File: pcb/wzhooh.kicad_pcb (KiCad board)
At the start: 2 copper layers, 1 part, among them U1 Pico

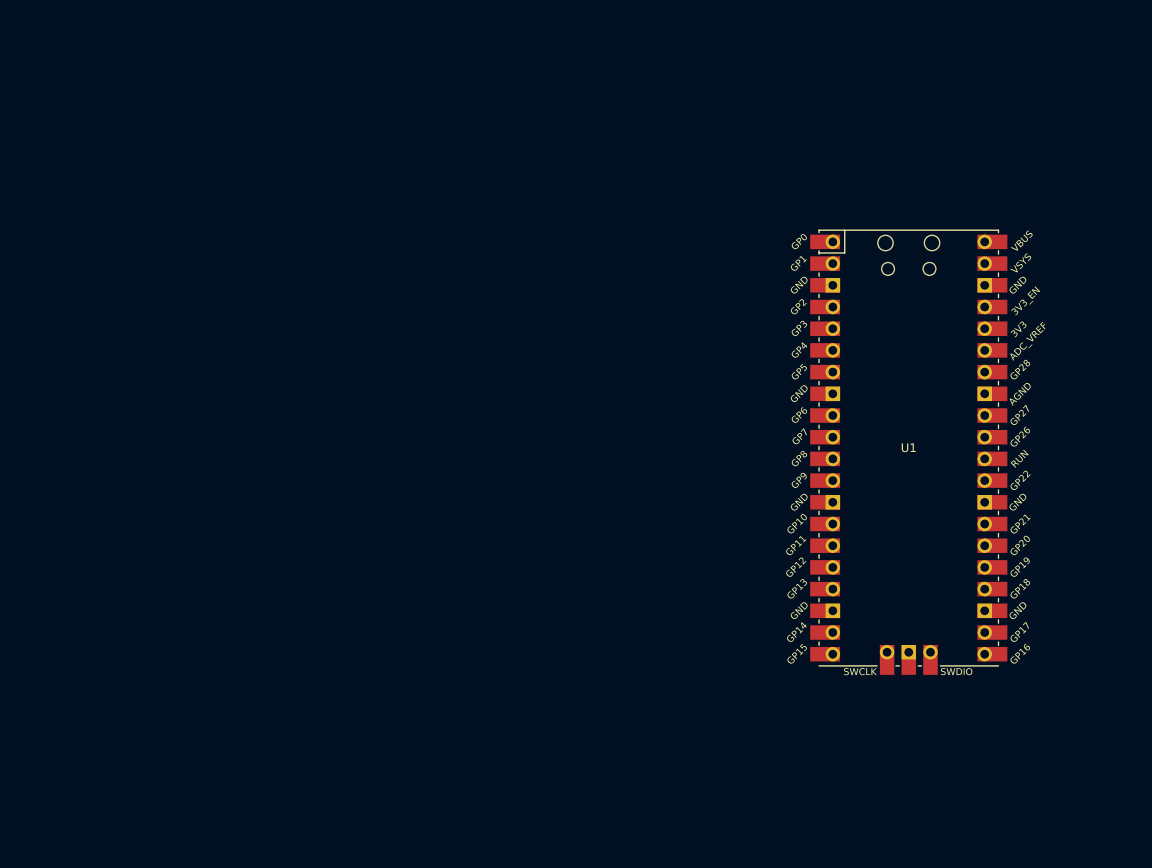
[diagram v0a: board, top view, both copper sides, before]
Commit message: rename project
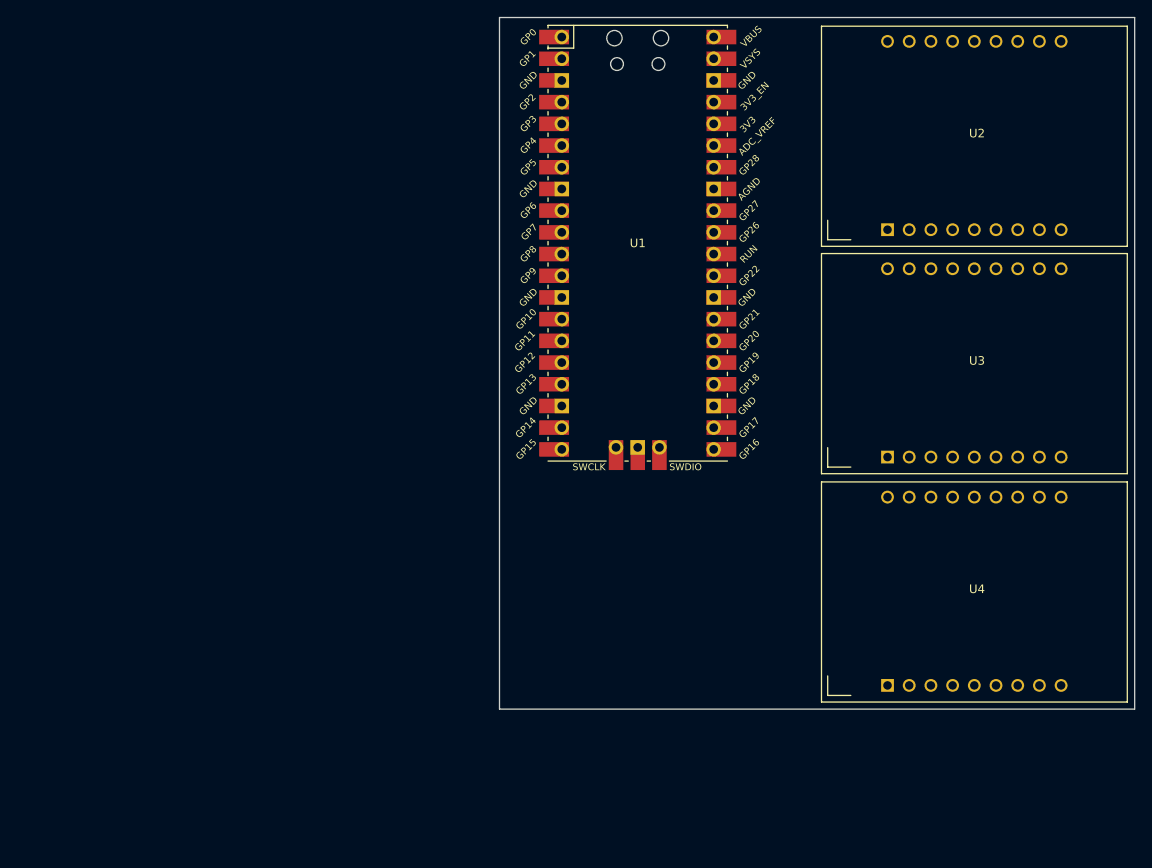
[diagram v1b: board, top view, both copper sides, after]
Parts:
- added U2: DA08-11SURKWA, Library:DA08-11, F.Cu at (150.1, 52.8)
- added U3: DA08-11SURKWA, Library:DA08-11, F.Cu at (150.1, 79.4)
- added U4: DA08-11SURKWA, Library:DA08-11, F.Cu at (150.1, 106.2)
- moved U1 39.8 mm to (110.7, 65.8)
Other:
- board outline added: 74.3 x 80.9 mm

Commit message: pcb rev:0x01
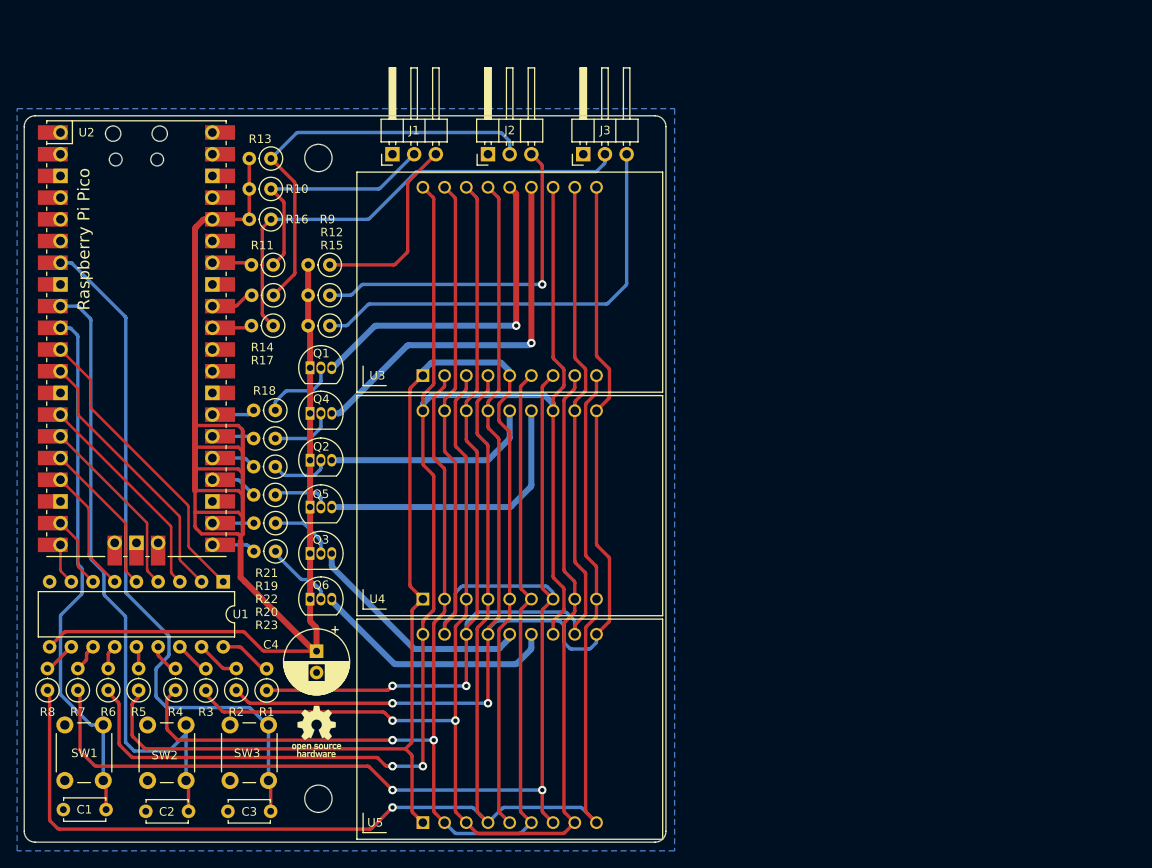
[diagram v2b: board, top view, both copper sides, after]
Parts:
- added C1: 1nF, Capacitor_THT:C_Disc_D4.7mm_W2.5mm_P5.00mm, F.Cu at (48.5, 132.1)
- added C2: 1nF, Capacitor_THT:C_Disc_D4.7mm_W2.5mm_P5.00mm, F.Cu at (58.2, 132.3)
- added C3: 1nF, Capacitor_THT:C_Disc_D4.7mm_W2.5mm_P5.00mm, F.Cu at (67.8, 132.3)
- added C4: 4.7uF, Capacitor_THT:CP_Radial_D7.5mm_P2.50mm, F.Cu at (73.2, 113.5)
- added H1: MountingHole, MountingHole:MountingHole_3.2mm_M3, F.Cu at (73.4, 55.8)
- added H2: MountingHole, MountingHole:MountingHole_3.2mm_M3, F.Cu at (73.4, 130.8)
- added J1: Sensor1, Connector_PinHeader_2.54mm:PinHeader_1x03_P2.54mm_Horizontal, F.Cu at (82.0, 55.4)
- added J2: Sensor2, Connector_PinHeader_2.54mm:PinHeader_1x03_P2.54mm_Horizontal, F.Cu at (93.2, 55.4)
- added J3: Sensor3, Connector_PinHeader_2.54mm:PinHeader_1x03_P2.54mm_Horizontal, F.Cu at (104.4, 55.4)
- added Q1: 2N3905, Package_TO_SOT_THT:TO-92_Inline, F.Cu at (72.4, 80.4)
- added Q2: 2N3905, Package_TO_SOT_THT:TO-92_Inline, F.Cu at (72.4, 91.2)
- added Q3: 2N3905, Package_TO_SOT_THT:TO-92_Inline, F.Cu at (72.4, 102.1)
- added Q4: 2N3905, Package_TO_SOT_THT:TO-92_Inline, F.Cu at (72.4, 85.7)
- added Q5: 2N3905, Package_TO_SOT_THT:TO-92_Inline, F.Cu at (72.4, 96.7)
- added Q6: 2N3905, Package_TO_SOT_THT:TO-92_Inline, F.Cu at (72.4, 107.4)
- added R1: 50Ω, Resistor_THT:R_Axial_DIN0207_L6.3mm_D2.5mm_P2.54mm_Vertical, F.Cu at (67.3, 118.1)
- added R10: 100KΩ, Resistor_THT:R_Axial_DIN0207_L6.3mm_D2.5mm_P2.54mm_Vertical, F.Cu at (67.8, 59.4)
- added R11: 330Ω, Resistor_THT:R_Axial_DIN0207_L6.3mm_D2.5mm_P2.54mm_Vertical, F.Cu at (68.1, 68.3)
- added R12: 330Ω, Resistor_THT:R_Axial_DIN0207_L6.3mm_D2.5mm_P2.54mm_Vertical, F.Cu at (74.7, 71.9)
- added R13: 100KΩ, Resistor_THT:R_Axial_DIN0207_L6.3mm_D2.5mm_P2.54mm_Vertical, F.Cu at (67.8, 55.9)
- added R14: 330Ω, Resistor_THT:R_Axial_DIN0207_L6.3mm_D2.5mm_P2.54mm_Vertical, F.Cu at (68.1, 71.9)
- added R15: 330Ω, Resistor_THT:R_Axial_DIN0207_L6.3mm_D2.5mm_P2.54mm_Vertical, F.Cu at (74.7, 75.4)
- added R16: 100KΩ, Resistor_THT:R_Axial_DIN0207_L6.3mm_D2.5mm_P2.54mm_Vertical, F.Cu at (67.8, 63.0)
- added R17: 330Ω, Resistor_THT:R_Axial_DIN0207_L6.3mm_D2.5mm_P2.54mm_Vertical, F.Cu at (68.1, 75.4)
- added R18: 330Ω, Resistor_THT:R_Axial_DIN0207_L6.3mm_D2.5mm_P2.54mm_Vertical, F.Cu at (68.3, 85.3)
- added R19: 330Ω, Resistor_THT:R_Axial_DIN0207_L6.3mm_D2.5mm_P2.54mm_Vertical, F.Cu at (68.3, 91.9)
- added R2: 50Ω, Resistor_THT:R_Axial_DIN0207_L6.3mm_D2.5mm_P2.54mm_Vertical, F.Cu at (63.8, 118.1)
- added R20: 330Ω, Resistor_THT:R_Axial_DIN0207_L6.3mm_D2.5mm_P2.54mm_Vertical, F.Cu at (68.4, 98.6)
- added R21: 330Ω, Resistor_THT:R_Axial_DIN0207_L6.3mm_D2.5mm_P2.54mm_Vertical, F.Cu at (68.3, 88.6)
- added R22: 330Ω, Resistor_THT:R_Axial_DIN0207_L6.3mm_D2.5mm_P2.54mm_Vertical, F.Cu at (68.3, 95.2)
- added R23: 330Ω, Resistor_THT:R_Axial_DIN0207_L6.3mm_D2.5mm_P2.54mm_Vertical, F.Cu at (68.4, 101.9)
- added R3: 50Ω, Resistor_THT:R_Axial_DIN0207_L6.3mm_D2.5mm_P2.54mm_Vertical, F.Cu at (60.2, 118.1)
- added R4: 50Ω, Resistor_THT:R_Axial_DIN0207_L6.3mm_D2.5mm_P2.54mm_Vertical, F.Cu at (56.6, 118.1)
- added R5: 50Ω, Resistor_THT:R_Axial_DIN0207_L6.3mm_D2.5mm_P2.54mm_Vertical, F.Cu at (52.3, 118.1)
- added R6: 50Ω, Resistor_THT:R_Axial_DIN0207_L6.3mm_D2.5mm_P2.54mm_Vertical, F.Cu at (48.8, 118.1)
- added R7: 50Ω, Resistor_THT:R_Axial_DIN0207_L6.3mm_D2.5mm_P2.54mm_Vertical, F.Cu at (45.2, 118.1)
- added R8: 50Ω, Resistor_THT:R_Axial_DIN0207_L6.3mm_D2.5mm_P2.54mm_Vertical, F.Cu at (41.7, 118.1)
- added R9: 330Ω, Resistor_THT:R_Axial_DIN0207_L6.3mm_D2.5mm_P2.54mm_Vertical, F.Cu at (74.7, 68.3)
- added REF**: OSHW-Logo_5.7x6mm_SilkScreen, Symbol:OSHW-Logo_5.7x6mm_SilkScreen, F.Cu at (73.2, 122.9)
- added SW1: Button1, Button_Switch_THT:SW_PUSH_6mm_H13mm, F.Cu at (43.7, 128.7)
- added SW2: Button2, Button_Switch_THT:SW_PUSH_6mm_H13mm, F.Cu at (53.4, 128.7)
- added SW3: Button3, Button_Switch_THT:SW_PUSH_6mm_H13mm, F.Cu at (63.0, 128.7)
- added U1: ULN2803A, Package_DIP:DIP-18_W7.62mm, F.Cu at (62.2, 105.4)
- moved U2 59.7 mm to (52.1, 77.0)
- moved U3 57.0 mm to (95.7, 69.9)
- moved U4 56.9 mm to (95.7, 96.1)
- moved U5 56.7 mm to (95.7, 122.2)
- renumbered U1 to U2, U2 to U3, U3 to U4, U4 to U5
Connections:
- U2 pad 10: unconnected-(U1-GPIO7-Pad10) -> /BTN_1
- U2 pad 11: unconnected-(U1-GPIO8-Pad11) -> Net-(U1-I1)
- U2 pad 12: unconnected-(U1-GPIO9-Pad12) -> Net-(U1-I2)
- U2 pad 13: unconnected-(U1-GND-Pad13) -> GND
- U2 pad 14: unconnected-(U1-GPIO10-Pad14) -> Net-(U1-I3)
- U2 pad 15: unconnected-(U1-GPIO11-Pad15) -> Net-(U1-I4)
- U2 pad 16: unconnected-(U1-GPIO12-Pad16) -> Net-(U1-I5)
- U2 pad 17: unconnected-(U1-GPIO13-Pad17) -> Net-(U1-I6)
- U2 pad 18: unconnected-(U1-GND-Pad18) -> GND
- U2 pad 19: unconnected-(U1-GPIO14-Pad19) -> Net-(U1-I7)
- U2 pad 20: unconnected-(U1-GPIO15-Pad20) -> Net-(U1-I8)
- U2 pad 21: unconnected-(U1-GPIO16-Pad21) -> /COM_6
- U2 pad 22: unconnected-(U1-GPIO17-Pad22) -> /COM_5
- U2 pad 23: unconnected-(U1-GND-Pad23) -> GND
- U2 pad 24: unconnected-(U1-GPIO18-Pad24) -> /COM_4
- U2 pad 25: unconnected-(U1-GPIO19-Pad25) -> /COM_3
- U2 pad 26: unconnected-(U1-GPIO20-Pad26) -> /COM_2
- U2 pad 27: unconnected-(U1-GPIO21-Pad27) -> /COM_1
- U2 pad 28: unconnected-(U1-GND-Pad28) -> GND
- U2 pad 3: unconnected-(U1-GND-Pad3) -> GND
- U2 pad 31: unconnected-(U1-GPIO26_ADC0-Pad31) -> /SENSE_3
- U2 pad 32: unconnected-(U1-GPIO27_ADC1-Pad32) -> /SENSE_2
- U2 pad 34: unconnected-(U1-GPIO28_ADC2-Pad34) -> /SENSE_1
- U2 pad 36: unconnected-(U1-3V3-Pad36) -> VDD
- U2 pad 38: unconnected-(U1-GND-Pad38) -> GND
- U2 pad 42: unconnected-(U1-GND-Pad42) -> GND
- U2 pad 7: unconnected-(U1-GPIO5-Pad7) -> /BTN_3
- U2 pad 8: unconnected-(U1-GND-Pad8) -> GND
- U2 pad 9: unconnected-(U1-GPIO6-Pad9) -> /BTN_2
- U3 pad 13: unconnected-(U2-DIG2_CA-Pad13) -> Net-(Q4-C)
- U3 pad 14: unconnected-(U2-DIG1_CA-Pad14) -> Net-(Q1-C)
- U4 pad 13: unconnected-(U3-DIG2_CA-Pad13) -> Net-(Q5-C)
- U4 pad 14: unconnected-(U3-DIG1_CA-Pad14) -> Net-(Q2-C)
- U5 pad 13: unconnected-(U4-DIG2_CA-Pad13) -> Net-(Q6-C)
- U5 pad 14: unconnected-(U4-DIG1_CA-Pad14) -> Net-(Q3-C)
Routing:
- net VDD: track 0.00 -> 193.7 mm
- net /SEG_DP: track 0.00 -> 191.6 mm, vias 0 -> 1
- net /SEG_G: track 0.00 -> 190.0 mm, vias 0 -> 2
- net /SEG_F: track 0.00 -> 185.1 mm, vias 0 -> 2
- net /SEG_B: track 0.00 -> 164.6 mm, vias 0 -> 2
- net /SEG_E: track 0.00 -> 159.7 mm
- net /SEG_D: track 0.00 -> 156.6 mm, vias 0 -> 2
- net /SEG_A: track 0.00 -> 154.7 mm, vias 0 -> 2
- net /SEG_C: track 0.00 -> 153.3 mm, vias 0 -> 2
- net /BTN_3: track 0.00 -> 81.7 mm
- net /BTN_2: track 0.00 -> 74.5 mm
- net /BTN_1: track 0.00 -> 61.6 mm
- net Net-(J3-Pin_2): track 0.00 -> 56.2 mm
- net Net-(J3-Pin_3): track 0.00 -> 51.9 mm
- net Net-(J2-Pin_2): track 0.00 -> 49.3 mm
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- added copper zone on B.Cu, net GND
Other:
- board size 74.3 x 80.9 mm -> 75.1 x 85 mm
- board text added: "LED SENSOR GND"
- board text added: "Raspberry Pi Pico"
- board text added: "Slot Car Lap Timer"
- board text added: "Track 1"
- board text added: "Track 2"
- board text added: "Track 3"
- board text added: "https://vitaly.codes/wzhooh | rev: 0x01"
- board text added: "Гурток трасового автомоделізму ЦНТТ {dblquote}Шанс{dblquote}, Вишневе, Київщина https://www.shanscentr.com.ua"

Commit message: rev: 0x01
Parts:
- C4: value 4.7uF -> 10uF
- Q1, Q2, Q3, Q4, Q5: value 2N3905 -> 2N2907
- R1, R2, R3, R4, R5, R6, R7, R8: value 50Ω -> 33Ω
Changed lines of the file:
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@@
         (effects (font (size 1 1) (thickness 0.15)))
     )
-    (fp_text value "50Ω" (at 1.27 2.37 90) (layer "F.Fab")
+    (fp_text value "33Ω" (at 1.27 2.37 90) (layer "F.Fab")
         (effects (font (size 1 1) (thickness 0.15)))
     )
@@
         (effects (font (size 1 1) (thickness 0.15)))
     )
-    (fp_text value "50Ω" (at 1.27 2.37 90) (layer "F.Fab")
+    (fp_text value "33Ω" (at 1.27 2.37 90) (layer "F.Fab")
         (effects (font (size 1 1) (thickness 0.15)))
     )
@@
         (effects (font (size 1 1) (thickness 0.15)))
     )
-    (fp_text value "50Ω" (at 1.27 2.37 90) (layer "F.Fab")
+    (fp_text value "33Ω" (at 1.27 2.37 90) (layer "F.Fab")
         (effects (font (size 1 1) (thickness 0.15)))
     )
@@
         (effects (font (size 1 1) (thickness 0.15)))
     )
-    (fp_text value "50Ω" (at 1.27 2.37 90) (layer "F.Fab")
+    (fp_text value "33Ω" (at 1.27 2.37 90) (layer "F.Fab")
         (effects (font (size 1 1) (thickness 0.15)))
     )
@@
         (effects (font (size 1 1) (thickness 0.15)))
     )
-    (fp_text value "50Ω" (at 1.27 2.37 90) (layer "F.Fab")
+    (fp_text value "33Ω" (at 1.27 2.37 90) (layer "F.Fab")
         (effects (font (size 1 1) (thickness 0.15)))
     )
@@
         (effects (font (size 1 1) (thickness 0.15)))
     )
-    (fp_text value "4.7uF" (at 1.25 5 -90) (layer "F.Fab")
+    (fp_text value "10uF" (at 1.25 5 -90) (layer "F.Fab")
         (effects (font (size 1 1) (thickness 0.15)))
     )
@@
         (effects (font (size 1 1) (thickness 0.15)))
     )
-    (fp_text value "2N3905" (at 1.27 2.79) (layer "F.Fab")
+    (fp_text value "2N2907" (at 1.27 2.79) (layer "F.Fab")
         (effects (font (size 1 1) (thickness 0.15)))
     )
@@
         (effects (font (size 1 1) (thickness 0.15)))
     )
-    (fp_text value "2N3905" (at 1.27 2.79) (layer "F.Fab")
+    (fp_text value "2N2907" (at 1.27 2.79) (layer "F.Fab")
         (effects (font (size 1 1) (thickness 0.15)))
     )
@@
         (effects (font (size 1 1) (thickness 0.15)))
     )
-    (fp_text value "50Ω" (at 1.27 2.37 90) (layer "F.Fab")
+    (fp_text value "33Ω" (at 1.27 2.37 90) (layer "F.Fab")
         (effects (font (size 1 1) (thickness 0.15)))
     )
@@
         (effects (font (size 1 1) (thickness 0.15)))
     )
-    (fp_text value "2N3905" (at 1.27 2.79) (layer "F.Fab")
+    (fp_text value "2N2907" (at 1.27 2.79) (layer "F.Fab")
         (effects (font (size 1 1) (thickness 0.15)))
     )
@@
         (effects (font (size 1 1) (thickness 0.15)))
     )
-    (fp_text value "50Ω" (at 1.27 2.37 90) (layer "F.Fab")
+    (fp_text value "33Ω" (at 1.27 2.37 90) (layer "F.Fab")
         (effects (font (size 1 1) (thickness 0.15)))
     )
@@
         (effects (font (size 1 1) (thickness 0.15)))
     )
-    (fp_text value "2N3905" (at 1.27 2.79) (layer "F.Fab")
+    (fp_text value "2N2907" (at 1.27 2.79) (layer "F.Fab")
         (effects (font (size 1 1) (thickness 0.15)))
     )
@@
         (effects (font (size 1 1) (thickness 0.15)))
     )
-    (fp_text value "50Ω" (at 1.27 2.37 90) (layer "F.Fab")
+    (fp_text value "33Ω" (at 1.27 2.37 90) (layer "F.Fab")
         (effects (font (size 1 1) (thickness 0.15)))
     )
@@
         (effects (font (size 1 1) (thickness 0.15)))
     )
-    (fp_text value "2N3905" (at 1.27 2.79) (layer "F.Fab")
+    (fp_text value "2N2907" (at 1.27 2.79) (layer "F.Fab")
         (effects (font (size 1 1) (thickness 0.15)))
     )
